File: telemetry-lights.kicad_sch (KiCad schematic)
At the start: 24 parts, among them J2 Conn_01x04, J3 Conn_01x03, J6 Conn_01x02, J8 Conn_01x02, U2 STM32L431KBU6TR, U3 IAM-20381HT

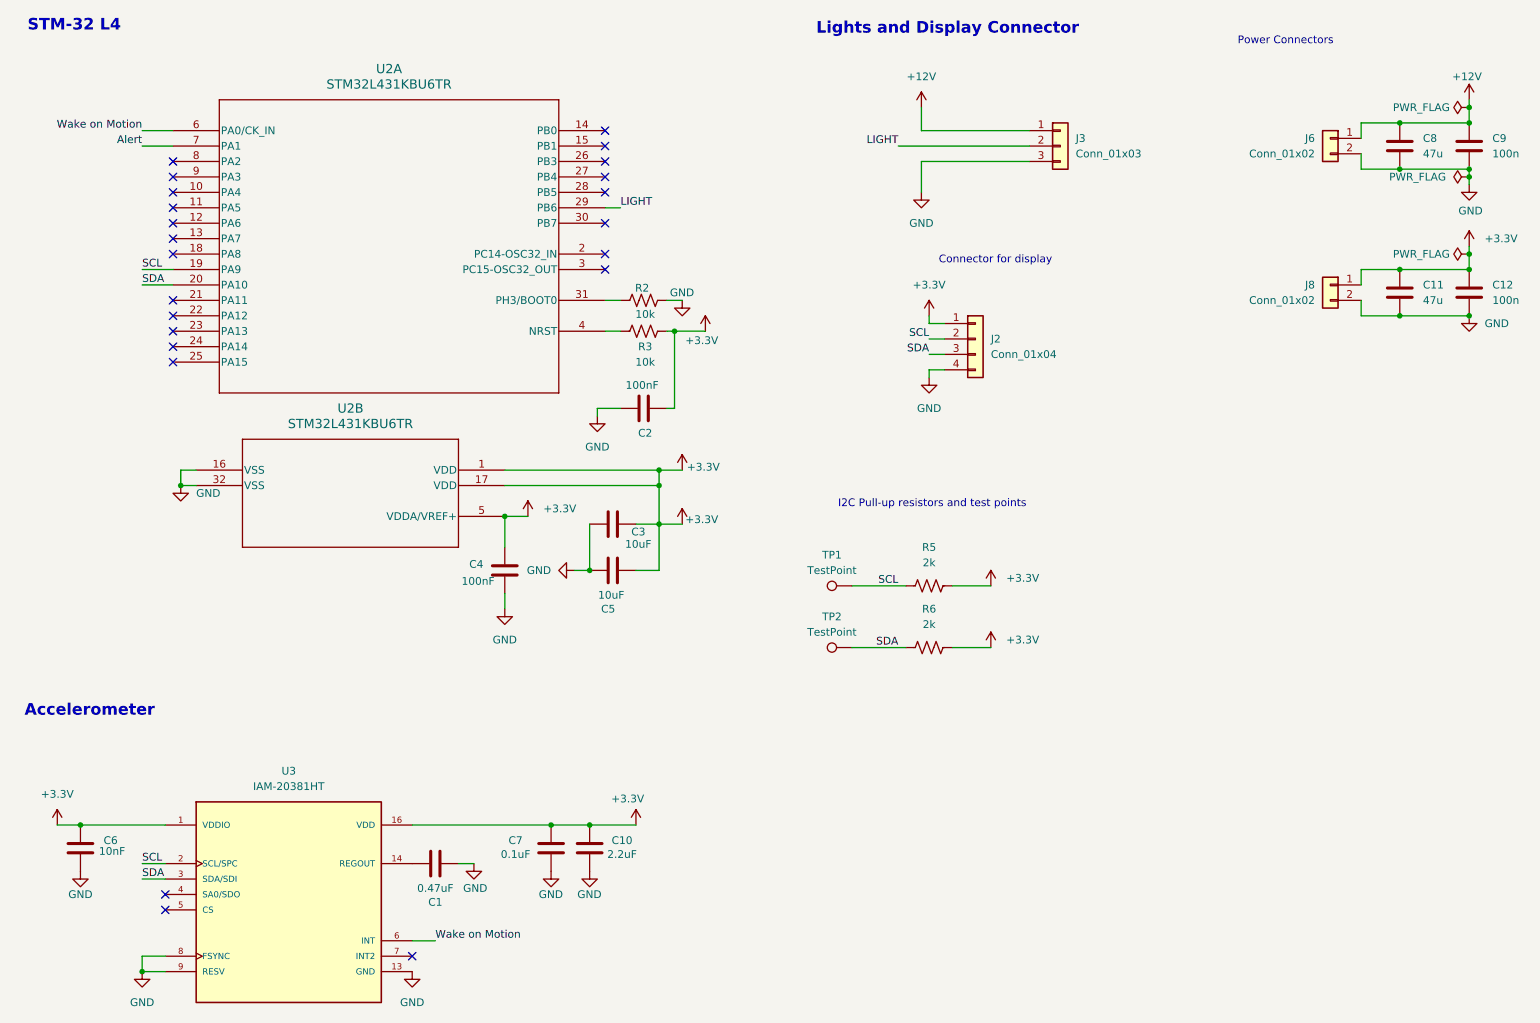
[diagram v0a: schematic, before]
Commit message: revised schematic
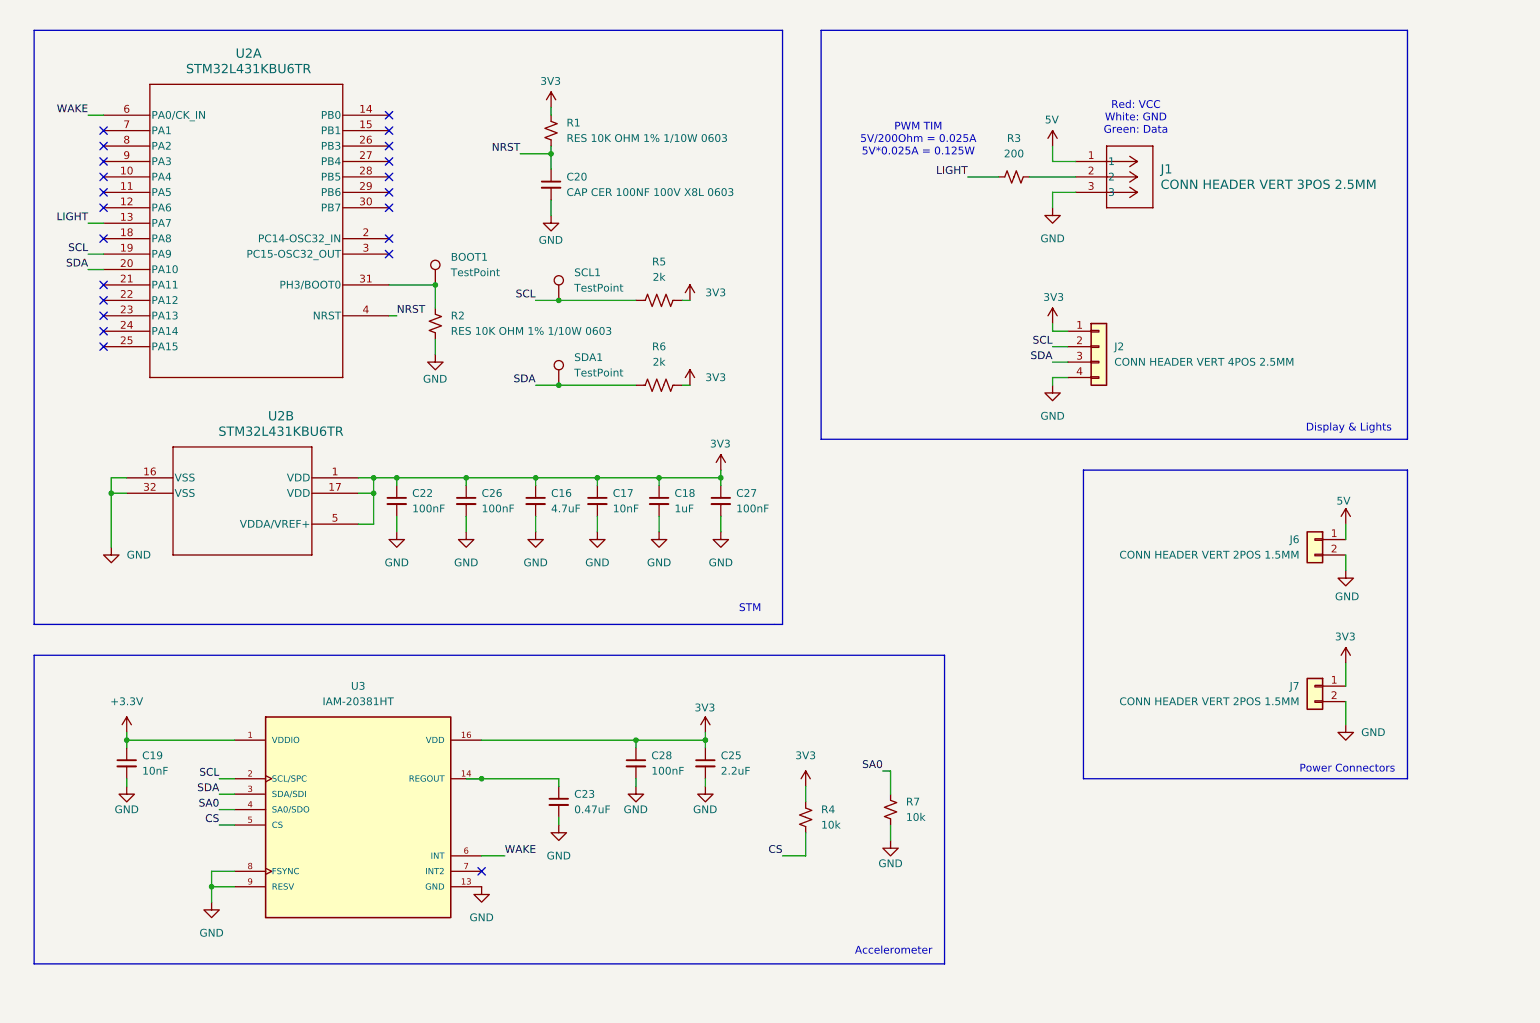
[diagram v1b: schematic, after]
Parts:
- removed C1: 0.47uF, Capacitor_SMD:C_0603_1608Metric_Pad1.08x0.95mm_HandSolder, symbol Device:C
- removed C10: 2.2uF, Capacitor_SMD:C_0603_1608Metric_Pad1.08x0.95mm_HandSolder, symbol Device:C
- removed C11, C8: 47u, Capacitor_SMD:C_0603_1608Metric_Pad1.08x0.95mm_HandSolder, symbol Device:C
- removed C12, C9: 100n, Capacitor_SMD:C_0603_1608Metric_Pad1.08x0.95mm_HandSolder, symbol Device:C
- removed C2, C4: 100nF, Capacitor_SMD:C_0603_1608Metric_Pad1.08x0.95mm_HandSolder, symbol Device:C
- removed C3, C5: 10uF, Capacitor_SMD:C_0603_1608Metric_Pad1.08x0.95mm_HandSolder, symbol Device:C
- removed C6: 10nF, symbol Device:C
- removed C7: 0.1uF, Capacitor_SMD:C_0603_1608Metric_Pad1.08x0.95mm_HandSolder, symbol Device:C
- removed J3: Conn_01x03, Connector_JST:JST_EH_B3B-EH-A_1x03_P2.50mm_Vertical, symbol Connector_Generic:Conn_01x03
- removed J8: Conn_01x02, Connector_JST:JST_PH_B2B-PH-K_1x02_P2.00mm_Vertical, symbol Connector_Generic:Conn_01x02
- removed R2, R3: 10k, Resistor_SMD:R_0603_1608Metric_Pad0.98x0.95mm_HandSolder, symbol Device:R_US
- added BOOT1: TestPoint, TestPoint:TestPoint_Pad_D1.0mm, symbol Connector:TestPoint
- added C16: 4.7uF, Capacitor_SMD:C_0603_1608Metric, symbol Device:C_Small
- added C17, C19: 10nF, Capacitor_SMD:C_0603_1608Metric, symbol Device:C_Small
- added C18: 1uF, Capacitor_SMD:C_0603_1608Metric, symbol Device:C_Small
- added C20: CAP CER 100NF 100V X8L 0603, Capacitor_SMD:C_0603_1608Metric, symbol Device:C_Small
- added C22, C26, C27, C28: 100nF, Capacitor_SMD:C_0603_1608Metric, symbol Device:C_Small
- added C23: 0.47uF, Capacitor_SMD:C_0603_1608Metric, symbol Device:C_Small
- added C25: 2.2uF, Capacitor_SMD:C_0603_1608Metric, symbol Device:C_Small
- added J1: CONN HEADER VERT 3POS 2.5MM, skateboard-footprint-library:CONN_B3B-XH-A_JST, symbol telemetry-lights:B3B-XH-A
- added J7: CONN HEADER VERT 2POS 1.5MM, Connector_JST:JST_ZH_B2B-ZR_1x02_P1.50mm_Vertical, symbol Connector_Generic:Conn_01x02
- added R1, R2: RES 10K OHM 1% 1/10W 0603, Resistor_SMD:R_0603_1608Metric, symbol Device:R_Small_US
- added R3: 200, Resistor_SMD:R_0603_1608Metric, symbol Device:R_Small_US
- added R4, R7: 10k, Resistor_SMD:R_0603_1608Metric, symbol Device:R_Small_US
- J2: value Conn_01x04 -> CONN HEADER VERT 4POS 2.5MM; footprint Connector_JST:JST_PH_B4B-PH-K_1x04_P2.00mm_Vertical -> Connector_JST:JST_EH_B4B-EH-A_1x04_P2.50mm_Vertical
- J6: value Conn_01x02 -> CONN HEADER VERT 2POS 1.5MM; footprint Connector_JST:JST_PH_B2B-PH-K_1x02_P2.00mm_Vertical -> Connector_JST:JST_ZH_B2B-ZR_1x02_P1.50mm_Vertical
- U2: footprint UFQFPN-32 -> skateboard-footprint-library:UFQFPN-32
- renumbered TP1 to SCL1, TP2 to SDA1
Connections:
- net +3.3V: now also C19.1; no longer J2.1 (Pin_1), R5.2, R6.2, U2.1 (VDD), U2.17 (VDD), U2.5 (VDDA/VREF+), U3.16 (VDD)
- net GND: now also C16.2, C17.2, C18.2, C19.2, C20.2, C22.2, C23.2, C25.2, C26.2, C27.2, C28.2, J1.3, J7.2 (Pin_2), R2.2, R7.2
- net LIGHT: now also U2.13 (PA7), R3.1; no longer U2.29 (PB6)
- net at U2.31 (PH3/BOOT0): now also BOOT1.1, R2.1
- net NRST: now reaches U2.4 (NRST)
- net NRST: now also C20.1, R1.2
- net at U3.14 (REGOUT): now also C23.1
- net SA0: now reaches U3.4 (SA0/SDO)
- net SA0: now also R7.1
- net CS: now reaches U3.5 (CS)
- net CS: now also R4.2
- net +12V renamed 5V
- net 5V: now also J1.1
- net Alert: no longer names the net of U2.7 (PA1)
- net Wake on Motion renamed WAKE
- new net: J1.2, R3.2
- new net 3V3: C16.1, C17.1, C18.1, C22.1, C25.1, C26.1, C27.1, C28.1, J2.1 (Pin_1), J7.1 (Pin_1), R1.1, R4.1, R5.2, R6.2, U2.1 (VDD), U2.17 (VDD), U2.5 (VDDA/VREF+), U3.16 (VDD)
- no-connect marks 23 -> 22
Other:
- note added: "Display & Lights"
- note added: "PWM TIM 5V/200Ohm = 0.025A 5V*0.025A = 0.125W"
- note added: "Red: VCC White: GND Green: Data"
- note added: "STM"
- note removed: "Connector for display"
- note removed: "I2C Pull-up resistors and test points"
- note removed: "Lights and Display Connector"
- note removed: "STM-32 L4"
- moved on the sheet: J2, J6, R5, SCL1, SDA1, U2A, U2B, U3
